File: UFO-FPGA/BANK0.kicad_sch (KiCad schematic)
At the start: 3 parts, among them U1 ICE40HX8K-BG121

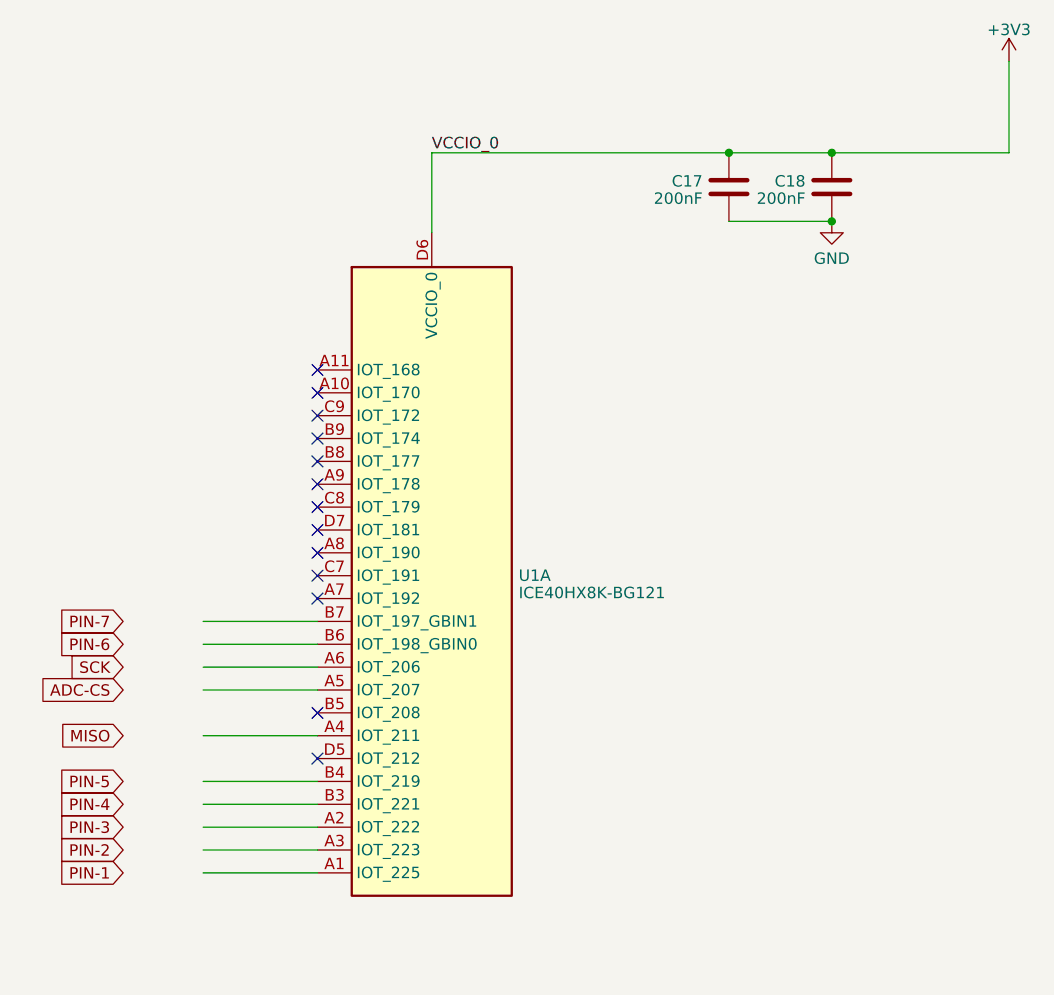
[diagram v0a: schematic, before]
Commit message: pcb
added John zendong
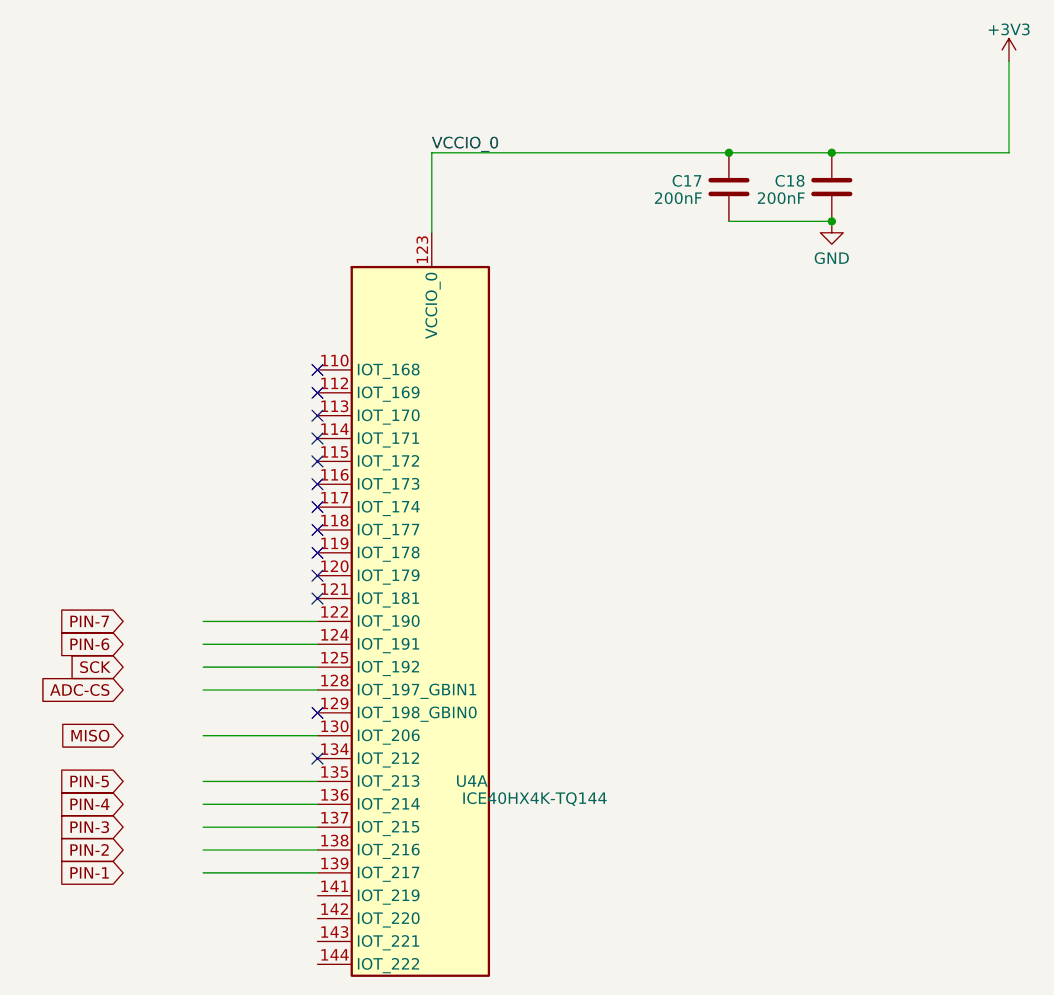
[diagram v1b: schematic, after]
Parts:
- removed U1: ICE40HX8K-BG121, Package_BGA:BGA-121_9.0x9.0mm_Layout11x11_P0.8mm_Ball0.4mm_Pad0.35mm_NSMD, symbol FPGA_Lattice:ICE40HX8K-BG121
- added U4: ICE40HX4K-TQ144, Package_QFP:TQFP-144_20x20mm_P0.5mm, symbol FPGA_Lattice:ICE40HX4K-TQ144
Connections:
- net +3V3: now also U4.123 (VCCIO_0), U4.131 (VCCIO_0)

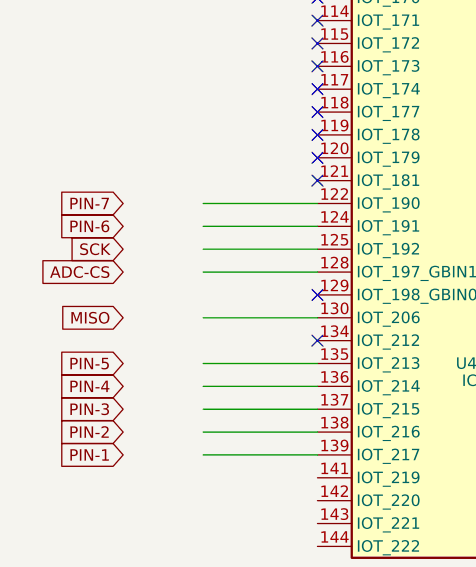
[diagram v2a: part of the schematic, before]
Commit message: pcb
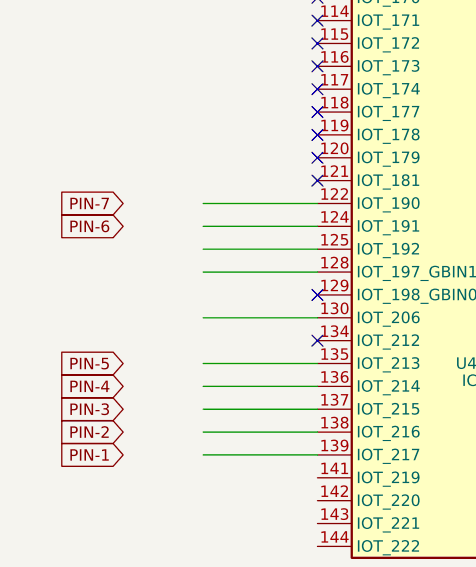
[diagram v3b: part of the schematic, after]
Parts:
- C17, C18: footprint Capacitor_SMD:C_0603_1608Metric_Pad1.08x0.95mm_HandSolder -> Capacitor_SMD:C_0805_2012Metric_Pad1.18x1.45mm_HandSolder
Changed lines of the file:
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@@
-    )
-  )
-  (global_label "MISO" (shape input) (at 92.71 113.665 180) (fields_autoplaced)
-    (effects (font (size 1.27 1.27)) (justify right))
-    (property "Intersheetrefs" "${INTERSHEET_REFS}" (at 85.208 113.665 0)
-      (effects (font (size 1.27 1.27)) (justify right) hide)
-    )
-  )
-  (global_label "ADC-CS" (shape input) (at 92.71 108.585 180) (fields_autoplaced)
-    (effects (font (size 1.27 1.27)) (justify right))
-    (property "Intersheetrefs" "${INTERSHEET_REFS}" (at 82.1237 108.585 0)
-      (effects (font (size 1.27 1.27)) (justify right) hide)
     )
   )
@@
     (effects (font (size 1.27 1.27)) (justify right))
     (property "Intersheetrefs" "${INTERSHEET_REFS}" (at 83.817 128.905 0)
-      (effects (font (size 1.27 1.27)) (justify right) hide)
-    )
-  )
-  (global_label "SCK" (shape input) (at 92.71 106.045 180) (fields_autoplaced)
-    (effects (font (size 1.27 1.27)) (justify right))
-    (property "Intersheetrefs" "${INTERSHEET_REFS}" (at 86.0547 106.045 0)
       (effects (font (size 1.27 1.27)) (justify right) hide)
     )
@@
       (effects (font (size 1.27 1.27)) (justify left))
     )
-    (property "Footprint" "Capacitor_SMD:C_0603_1608Metric_Pad1.08x0.95mm_HandSolder" (at 159.0548 56.515 0)
+    (property "Footprint" "Capacitor_SMD:C_0805_2012Metric_Pad1.18x1.45mm_HandSolder" (at 159.0548 56.515 0)
       (effects (font (size 1.27 1.27)) hide)
     )
@@
       (effects (font (size 1.27 1.27)) (justify left))
     )
-    (property "Footprint" "Capacitor_SMD:C_0603_1608Metric_Pad1.08x0.95mm_HandSolder" (at 170.4848 56.515 0)
-      (effects (font (size 1.27 1.27)) hide)
-    )
+    (property "Footprint" "Capacitor_SMD:C_0805_2012Metric_Pad1.18x1.45mm_HandSolder" (at 170.4848 56.515 0)
+      (effects (font (size 1.27 1.27)) hide)
+    )

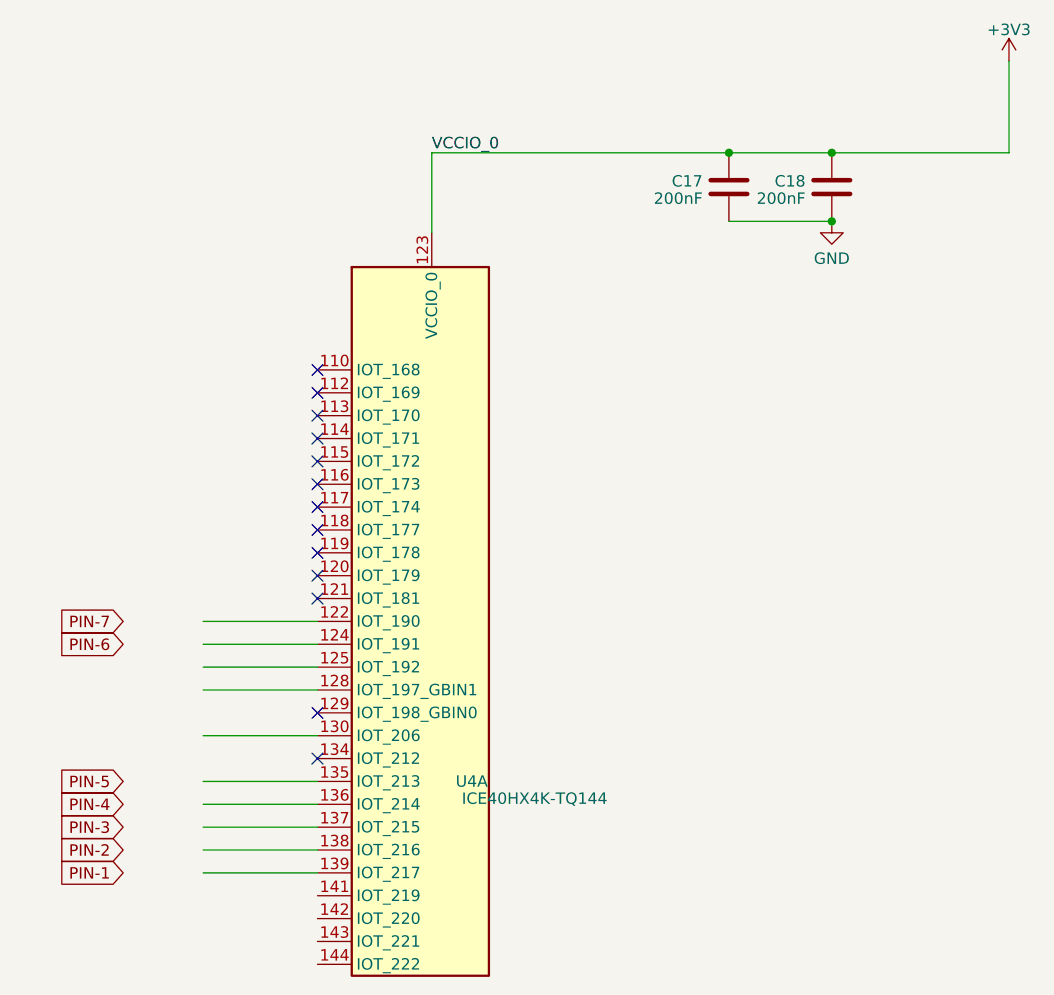
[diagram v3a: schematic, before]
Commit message: pcb
added monkey
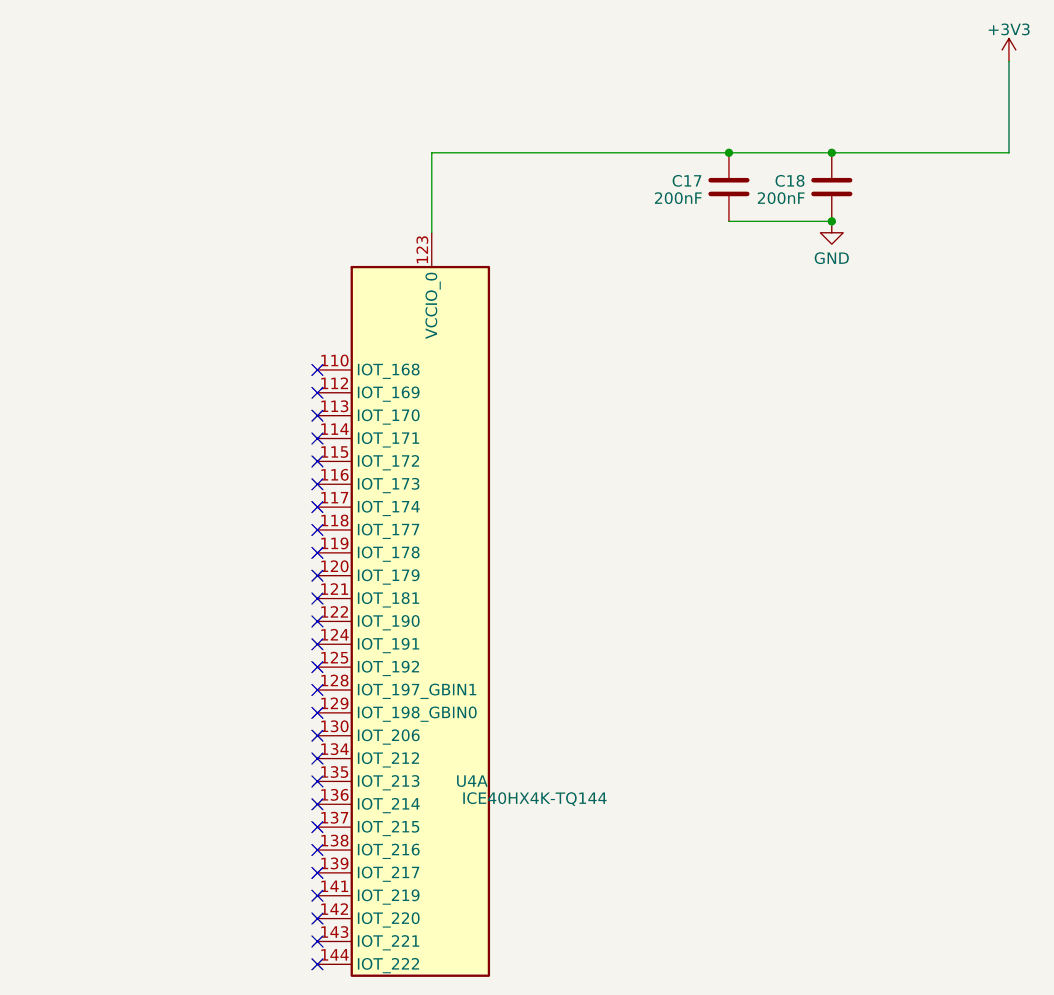
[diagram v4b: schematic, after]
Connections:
- no-connect marks 13 -> 27
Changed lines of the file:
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@@
   (junction (at 171.45 48.895) (diameter 0) (color 0 0 0 0)
   )
+  (no_connect (at 114.3 100.965))
+  (no_connect (at 114.3 126.365))
   (no_connect (at 114.3 90.805))
   (no_connect (at 114.3 85.725))
+  (no_connect (at 114.3 128.905))
+  (no_connect (at 114.3 106.045))
+  (no_connect (at 114.3 123.825))
+  (no_connect (at 114.3 108.585))
+  (no_connect (at 114.3 136.525))
+  (no_connect (at 114.3 133.985))
+  (no_connect (at 114.3 118.745))
   (no_connect (at 114.3 111.125))
   (no_connect (at 114.3 93.345))
@@
   (no_connect (at 114.3 98.425))
   (no_connect (at 114.3 73.025))
+  (no_connect (at 114.3 121.285))
   (no_connect (at 114.3 75.565))
+  (no_connect (at 114.3 131.445))
   (no_connect (at 114.3 80.645))
+  (no_connect (at 114.3 139.065))
+  (no_connect (at 114.3 103.505))
   (no_connect (at 114.3 83.185))
   (no_connect (at 114.3 116.205))
+  (no_connect (at 114.3 113.665))
   (no_connect (at 114.3 95.885))
   (no_connect (at 114.3 88.265))
-  (wire (pts (xy 101.6 118.745) (xy 114.3 118.745))
-    (stroke (width 0) (type default))
-  )
-  (wire (pts (xy 101.6 128.905) (xy 114.3 128.905))
-    (stroke (width 0) (type default))
-  )
   (wire (pts (xy 191.135 48.895) (xy 191.135 38.735))
-    (stroke (width 0) (type default))
-  )
-  (wire (pts (xy 101.6 100.965) (xy 114.3 100.965))
-    (stroke (width 0) (type default))
-  )
-  (wire (pts (xy 101.6 108.585) (xy 114.3 108.585))
     (stroke (width 0) (type default))
   )
@@
     (stroke (width 0) (type default))
   )
-  (wire (pts (xy 101.6 113.665) (xy 114.3 113.665))
-    (stroke (width 0) (type default))
-  )
   (wire (pts (xy 171.45 48.895) (xy 191.135 48.895))
-    (stroke (width 0) (type default))
-  )
-  (wire (pts (xy 101.6 121.285) (xy 114.3 121.285))
-    (stroke (width 0) (type default))
-  )
-  (wire (pts (xy 101.6 103.505) (xy 114.3 103.505))
-    (stroke (width 0) (type default))
-  )
-  (wire (pts (xy 101.6 126.365) (xy 114.3 126.365))
     (stroke (width 0) (type default))
   )
@@
     (stroke (width 0) (type default))
   )
-  (wire (pts (xy 101.6 123.825) (xy 114.3 123.825))
-    (stroke (width 0) (type default))
-  )
-  (wire (pts (xy 101.6 106.045) (xy 114.3 106.045))
-    (stroke (width 0) (type default))
-  )
-  (label "VCCIO_0" (at 127 48.895 0) (fields_autoplaced)
-    (effects (font (size 1.27 1.27)) (justify left bottom))
-  )
-  (global_label "PIN-7" (shape input) (at 92.71 100.965 180) (fields_autoplaced)
-    (effects (font (size 1.27 1.27)) (justify right))
-    (property "Intersheetrefs" "${INTERSHEET_REFS}" (at 83.817 100.965 0)
-      (effects (font (size 1.27 1.27)) (justify right) hide)
-    )
-  )
-  (global_label "PIN-3" (shape input) (at 92.71 123.825 180) (fields_autoplaced)
-    (effects (font (size 1.27 1.27)) (justify right))
-    (property "Intersheetrefs" "${INTERSHEET_REFS}" (at 83.817 123.825 0)
-      (effects (font (size 1.27 1.27)) (justify right) hide)
-    )
-  )
-  (global_label "PIN-6" (shape input) (at 92.71 103.505 180) (fields_autoplaced)
-    (effects (font (size 1.27 1.27)) (justify right))
-    (property "Intersheetrefs" "${INTERSHEET_REFS}" (at 83.817 103.505 0)
-      (effects (font (size 1.27 1.27)) (justify right) hide)
-    )
-  )
-  (global_label "PIN-5" (shape input) (at 92.71 118.745 180) (fields_autoplaced)
-    (effects (font (size 1.27 1.27)) (justify right))
-    (property "Intersheetrefs" "${INTERSHEET_REFS}" (at 83.817 118.745 0)
-      (effects (font (size 1.27 1.27)) (justify right) hide)
-    )
-  )
-  (global_label "PIN-2" (shape input) (at 92.71 126.365 180) (fields_autoplaced)
-    (effects (font (size 1.27 1.27)) (justify right))
-    (property "Intersheetrefs" "${INTERSHEET_REFS}" (at 83.817 126.365 0)
-      (effects (font (size 1.27 1.27)) (justify right) hide)
-    )
-  )
-  (global_label "PIN-1" (shape input) (at 92.71 128.905 180) (fields_autoplaced)
-    (effects (font (size 1.27 1.27)) (justify right))
-    (property "Intersheetrefs" "${INTERSHEET_REFS}" (at 83.817 128.905 0)
-      (effects (font (size 1.27 1.27)) (justify right) hide)
-    )
-  )
-  (global_label "PIN-4" (shape input) (at 92.71 121.285 180) (fields_autoplaced)
-    (effects (font (size 1.27 1.27)) (justify right))
-    (property "Intersheetrefs" "${INTERSHEET_REFS}" (at 83.817 121.285 0)
-      (effects (font (size 1.27 1.27)) (justify right) hide)
-    )
-  )
   (symbol (lib_id "power:GND") (at 171.45 56.515 0) (unit 1)
